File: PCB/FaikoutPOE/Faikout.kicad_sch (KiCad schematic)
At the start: 85 parts, among them J1 RJ45_LED, J3 S21, J5 Reset, J7 TC2030-USB-NL-DS, M1 Ag9912-LP, P1 Square, Q1 BSS138PS, Q2 BSS138PS, U1 KSZ8851SNL, U2 ESP32-S3-MINI-1, U3 TCMT1100, U4 TPS62933, U5 TCMT1100, Y1 Crystal_GND24

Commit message: Re-render, latest layout
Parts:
- R10, R17: MPN (none) -> C270365
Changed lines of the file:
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@@
 			)
 		)
+		(property "MPN" "C270365"
+			(at 190.5 134.62 90)
+			(hide yes)
+			(show_name no)
+			(do_not_autoplace no)
+			(effects
+				(font
+					(size 1.27 1.27)
+				)
+			)
+		)
 		(pin "1"
 		)
@@
 			(hide yes)
 			(show_name no)
+			(do_not_autoplace no)
+			(effects
+				(font
+					(size 1.27 1.27)
+				)
+			)
+		)
+		(property "MPN" "C270365"
+			(at 213.36 134.62 90)
+			(hide yes)
+			(show_name no)

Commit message: Fix BOM
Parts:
- R18, R19: MPN C7467262 -> C138135
- R9: MPN C102690 -> C106225
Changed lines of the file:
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@@
 			)
 		)
-		(property "MPN" "C7467262"
+		(property "MPN" "C138135"
 			(at 31.75 58.42 90)
 			(hide yes)
@@
 			)
 		)
-		(property "MPN" "C7467262"
+		(property "MPN" "C138135"
 			(at 25.4 58.42 90)
 			(hide yes)
@@
 		(in_bom no)
 		(on_board yes)
-		(in_pos_files yes)
+		(in_pos_files no)
 		(dnp no)
 		(fields_autoplaced yes)
@@
 			)
 		)
-		(property "MPN" "C102690"
+		(property "MPN" "C106225"
 			(at 274.32 76.2 90)
 			(hide yes)

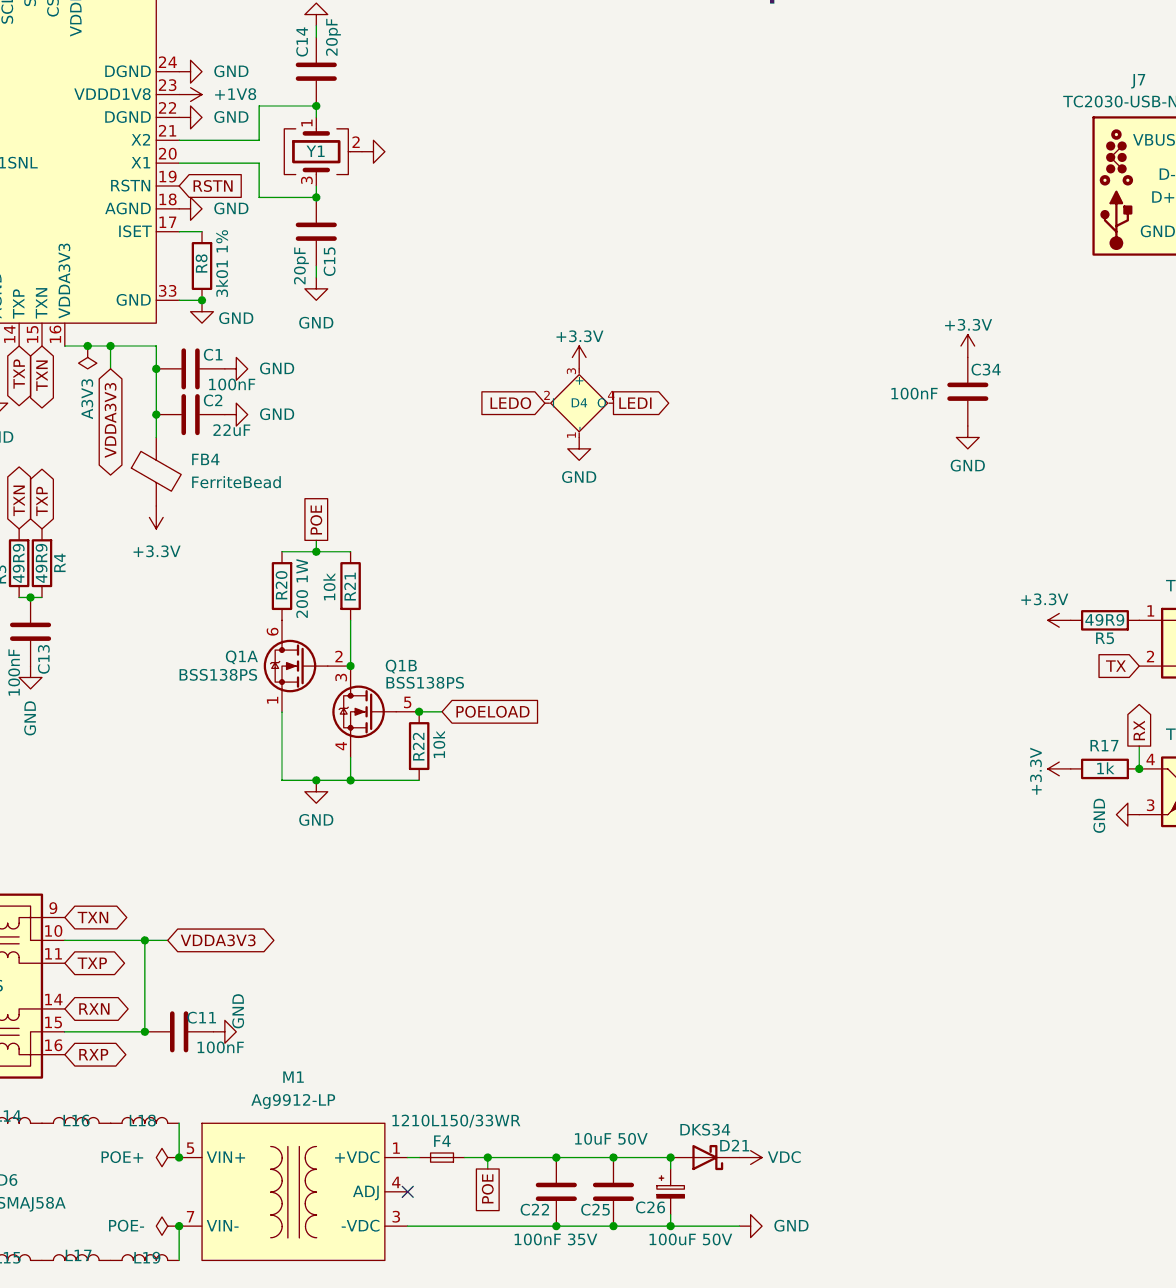
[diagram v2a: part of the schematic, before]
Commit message: Latest tweaks
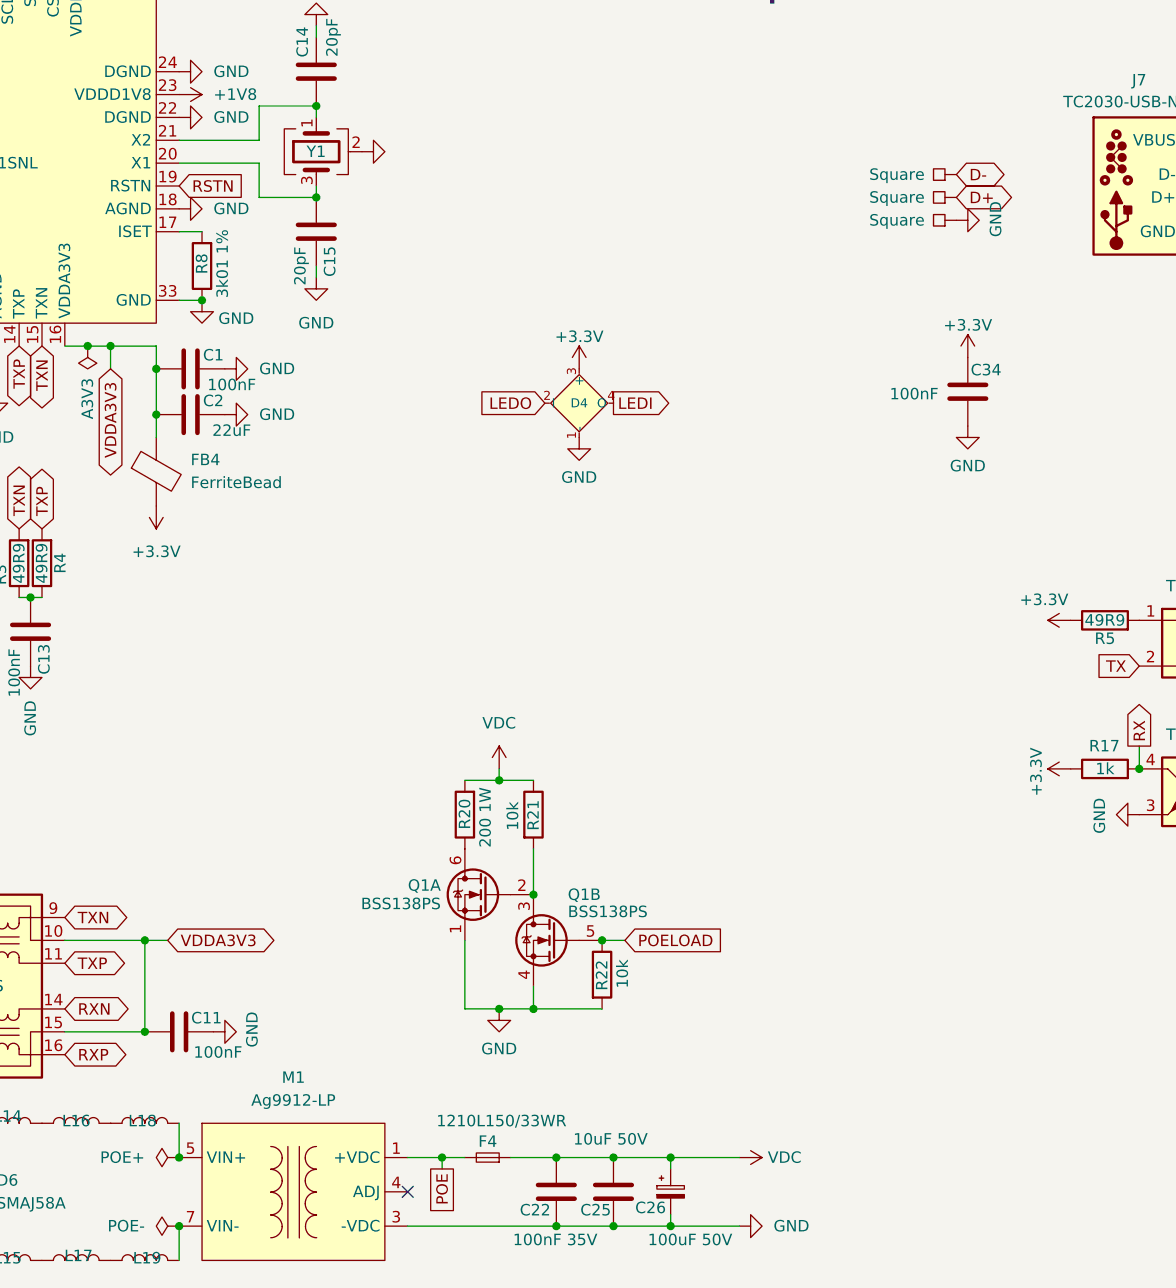
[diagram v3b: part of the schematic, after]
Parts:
- removed D21: DKS34, RevK:D_SOD-123FL, symbol Device:D_Schottky
- added P2, P3, P4: Square, RevK:PAD-2mm, symbol RevK:Square
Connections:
- net D+: now also P3.1 (P)
- net D-: now also P2.1 (P)
- net GND: now also P4.1 (P)
- net POE: now also F4.2, M1.1 (+VDC), M1.2 (+VDC); no longer C22.1, C25.2, C26.1, F4.1, R20.2, R21.1
- net VDC: now also C22.1, C25.2, C26.1, F4.1, R20.2, R21.1
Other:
- moved on the sheet: F4, Q1A, Q1B, R20, R21, R22
